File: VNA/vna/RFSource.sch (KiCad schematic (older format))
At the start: 15 parts, among them U4 AD9851, X1 30MHz

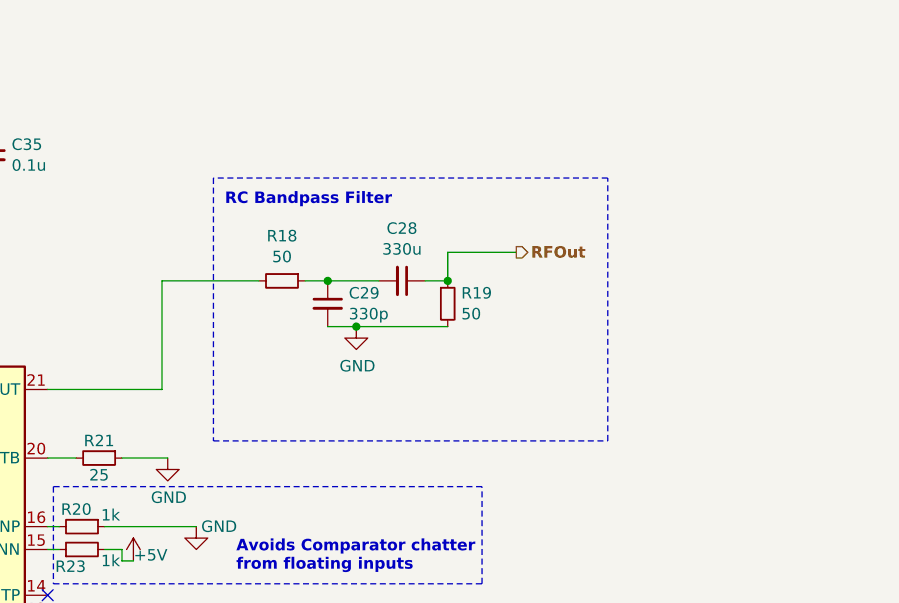
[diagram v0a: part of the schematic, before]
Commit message: v0.1 completed, producing gerbers
gerbers to be sent to jlc pcb pending their acceptance, they will be produced
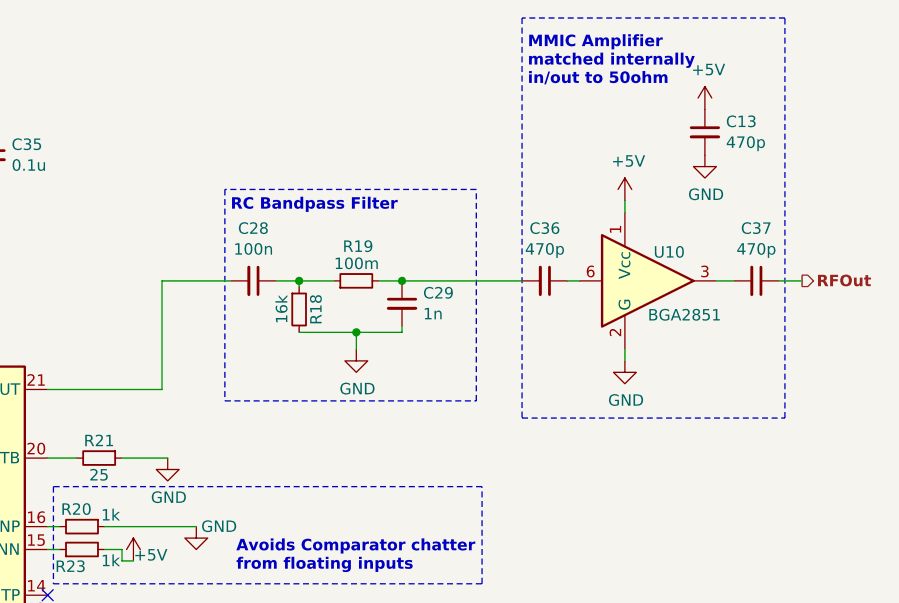
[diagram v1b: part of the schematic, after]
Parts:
- added C13, C36, C37: 470p, Capacitor_SMD:C_0805_2012Metric_Pad1.15x1.40mm_HandSolder, symbol Device:C_Small
- added U10: BGA2851, Package_TO_SOT_SMD:SOT-363_SC-70-6, symbol RF_Amplifier:BGA2851
- C28: value 330u -> 100n
- C29: value 330p -> 1n
- R18: value 50 -> 16k
- R19: value 50 -> 100m
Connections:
- net +5V: now also C13.1, U10.1 (Vcc)
- net GND: now also R18.2, C13.2, U10.2 (G), U10.4 (G), U10.5 (G); no longer R19.2
- net RFOut: now also C37.1; no longer C28.1, R19.1
- net at U4.21 (IOUT): now also C28.2; no longer R18.2
- new net: C28.1, R18.1, R19.1
- new net: C29.1, C36.2, R19.2
- new net: C37.2, U10.3
- new net: C36.1, U10.6
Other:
- note added: "MMIC Amplifier\nmatched internally\nin/out to 50ohm"
- moved on the sheet: C28, C29, R18, R19
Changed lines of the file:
@@
 Comment4 ""
 $EndDescr
-Text HLabel 6900 3400 2    50   Output ~ 10
+Text HLabel 8150 3525 2    50   Output ~ 10
 RFOut
 Text HLabel 3500 4900 0    50   Input ~ 10
@@
 Wire Wire Line
 	5350 4000 5350 3525
-Text Notes 5625 3200 0    50   ~ 10
+Text Notes 5650 3225 0    50   ~ 10
 RC Bandpass Filter
 $Comp
 L power:GND #PWR0102
 U 1 1 5D858459
-P 6200 3725
-F 0 "#PWR0102" H 6200 3475 50  0001 C CNN
-F 1 "GND" H 6205 3552 50  0000 C CNN
-F 2 "" H 6200 3725 50  0001 C CNN
-F 3 "" H 6200 3725 50  0001 C CNN
-	1    6200 3725
+P 6200 3825
+F 0 "#PWR0102" H 6200 3575 50  0001 C CNN
+F 1 "GND" H 6205 3652 50  0000 C CNN
+F 2 "" H 6200 3825 50  0001 C CNN
+F 3 "" H 6200 3825 50  0001 C CNN
+	1    6200 3825
 	1    0    0    -1
 $EndComp
@@
 L Device:R_Small R18
 U 1 1 5D90E295
-P 5875 3525
-F 0 "R18" V 5679 3525 50  0000 C CNN
-F 1 "50" V 5770 3525 50  0000 C CNN
-F 2 "Resistor_SMD:R_0805_2012Metric_Pad1.15x1.40mm_HandSolder" H 5875 3525 50  0001 C CNN
-F 3 "~" H 5875 3525 50  0001 C CNN
-	1    5875 3525
-	0    1    1    0
+P 5950 3650
+F 0 "R18" V 6025 3650 50  0000 C CNN
+F 1 "16k" V 5875 3650 50  0000 C CNN
+F 2 "Resistor_SMD:R_0805_2012Metric_Pad1.15x1.40mm_HandSolder" H 5950 3650 50  0001 C CNN
+F 3 "~" H 5950 3650 50  0001 C CNN
+	1    5950 3650
+	1    0    0    -1
 $EndComp
 $Comp
 L Device:R_Small R19
 U 1 1 5D90EC5A
-P 6600 3625
-F 0 "R19" H 6659 3671 50  0000 L CNN
-F 1 "50" H 6659 3580 50  0000 L CNN
-F 2 "Resistor_SMD:R_0805_2012Metric_Pad1.15x1.40mm_HandSolder" H 6600 3625 50  0001 C CNN
-F 3 "~" H 6600 3625 50  0001 C CNN
-	1    6600 3625
-	1    0    0    -1
+P 6200 3525
+F 0 "R19" V 6350 3450 50  0000 L CNN
+F 1 "100m" V 6275 3425 50  0000 L CNN
+F 2 "Resistor_SMD:R_0805_2012Metric_Pad1.15x1.40mm_HandSolder" H 6200 3525 50  0001 C CNN
+F 3 "~" H 6200 3525 50  0001 C CNN
+	1    6200 3525
+	0    -1   -1   0
 $EndComp
 $Comp
 L Device:C_Small C29
 U 1 1 5D90F928
-P 6075 3625
-F 0 "C29" H 6167 3671 50  0000 L CNN
-F 1 "330p" H 6167 3580 50  0000 L CNN
-F 2 "Capacitor_SMD:C_0805_2012Metric_Pad1.15x1.40mm_HandSolder" H 6075 3625 50  0001 C CNN
-F 3 "~" H 6075 3625 50  0001 C CNN
-	1    6075 3625
+P 6400 3625
+F 0 "C29" H 6492 3671 50  0000 L CNN
+F 1 "1n" H 6492 3580 50  0000 L CNN
+F 2 "Capacitor_SMD:C_0805_2012Metric_Pad1.15x1.40mm_HandSolder" H 6400 3625 50  0001 C CNN
+F 3 "~" H 6400 3625 50  0001 C CNN
+	1    6400 3625
 	1    0    0    -1
 $EndComp
@@
 L Device:C_Small C28
 U 1 1 5D9103E4
-P 6400 3525
-F 0 "C28" V 6171 3525 50  0000 C CNN
-F 1 "330u" V 6262 3525 50  0000 C CNN
-F 2 "Capacitor_SMD:C_0805_2012Metric_Pad1.15x1.40mm_HandSolder" H 6400 3525 50  0001 C CNN
-F 3 "~" H 6400 3525 50  0001 C CNN
-	1    6400 3525
+P 5750 3525
+F 0 "C28" V 5521 3525 50  0000 C CNN
+F 1 "100n" V 5612 3525 50  0000 C CNN
+F 2 "Capacitor_SMD:C_0805_2012Metric_Pad1.15x1.40mm_HandSolder" H 5750 3525 50  0001 C CNN
+F 3 "~" H 5750 3525 50  0001 C CNN
+	1    5750 3525
 	0    1    1    0
 $EndComp
-Wire Wire Line
-	5350 3525 5775 3525
-Wire Wire Line
-	5975 3525 6075 3525
-Wire Wire Line
-	6075 3525 6300 3525
-Connection ~ 6075 3525
-Wire Wire Line
-	6500 3525 6600 3525
-Wire Wire Line
-	6075 3725 6200 3725
-Connection ~ 6200 3725
-Wire Wire Line
-	6200 3725 6600 3725
-Wire Wire Line
-	6600 3525 6600 3400
-Wire Wire Line
-	6600 3400 6900 3400
-Connection ~ 6600 3525
-Wire Notes Line
-	5575 3075 5575 4225
-Wire Notes Line
-	5575 4225 7300 4225
-Wire Notes Line
-	7300 4225 7300 3075
-Wire Notes Line
-	7300 3075 5575 3075
 $Comp
 L Device:R_Small R20
@@
 Connection ~ 3550 2875
 Connection ~ 3550 3075
+$Comp
+L RF_Amplifier:BGA2851 U10
+U 1 1 5D98BDCA
+P 7475 3525
+F 0 "U10" H 7500 3650 50  0000 L CNN
+F 1 "BGA2851" H 7475 3375 50  0000 L CNN
+F 2 "Package_TO_SOT_SMD:SOT-363_SC-70-6" H 7425 2875 50  0001 C CNN
+F 3 "https://www.nxp.com/docs/en/data-sheet/BGA2851.pdf" H 7475 3525 50  0001 C CNN
+	1    7475 3525
+	1    0    0    -1
+$EndComp
+$Comp
+L power:+5V #PWR0120
+U 1 1 5D98ED21
+P 7375 3175
+F 0 "#PWR0120" H 7375 3025 50  0001 C CNN
+F 1 "+5V" H 7390 3348 50  0000 C CNN
+F 2 "" H 7375 3175 50  0001 C CNN
+F 3 "" H 7375 3175 50  0001 C CNN
+	1    7375 3175
+	1    0    0    -1
+$EndComp
+$Comp
+L power:GND #PWR0121
+U 1 1 5D98FE3B
+P 7375 3875
+F 0 "#PWR0121" H 7375 3625 50  0001 C CNN
+F 1 "GND" H 7380 3702 50  0000 C CNN
+F 2 "" H 7375 3875 50  0001 C CNN
+F 3 "" H 7375 3875 50  0001 C CNN
+	1    7375 3875
+	1    0    0    -1
+$EndComp
+Text Notes 6950 2675 0    50   ~ 10
+MMIC Amplifier\nmatched internally\nin/out to 50ohm
+Wire Wire Line
+	5350 3525 5650 3525
+Wire Wire Line
+	5850 3525 5950 3525
+Wire Wire Line
+	5950 3550 5950 3525
+Connection ~ 5950 3525
+Wire Wire Line
+	5950 3525 6100 3525
+Wire Wire Line
+	6300 3525 6400 3525
+Wire Wire Line
+	5950 3750 6200 3750
+Wire Wire Line
+	6400 3750 6400 3725
+Wire Wire Line
+	6200 3750 6200 3825
+Connection ~ 6200 3750
+Wire Wire Line
+	6200 3750 6400 3750
+Wire Notes Line
+	5625 3125 5625 4050
+Wire Notes Line
+	5625 4050 6725 4050
+Wire Notes Line
+	6725 4050 6725 3125
+Wire Notes Line
+	6725 3125 5625 3125
+Wire Wire Line
+	7375 3825 7375 3875
+Wire Wire Line
+	7375 3225 7375 3175
+$Comp
+L Device:C_Small C37
+U 1 1 5D9C2425
+P 7950 3525
+F 0 "C37" V 7721 3525 50  0000 C CNN
+F 1 "470p" V 7812 3525 50  0000 C CNN
+F 2 "Capacitor_SMD:C_0805_2012Metric_Pad1.15x1.40mm_HandSolder" H 7950 3525 50  0001 C CNN
+F 3 "~" H 7950 3525 50  0001 C CNN
+	1    7950 3525
+	0    1    1    0
+$EndComp
+$Comp
+L Device:C_Small C36
+U 1 1 5D9C3B15
+P 7025 3525
+F 0 "C36" V 6796 3525 50  0000 C CNN
+F 1 "470p" V 6887 3525 50  0000 C CNN
+F 2 "Capacitor_SMD:C_0805_2012Metric_Pad1.15x1.40mm_HandSolder" H 7025 3525 50  0001 C CNN
+F 3 "~" H 7025 3525 50  0001 C CNN
+	1    7025 3525
+	0    1    1    0
+$EndComp
+$Comp
+L Device:C_Small C13
+U 1 1 5D9C4738
+P 7725 2875
+F 0 "C13" H 7817 2921 50  0000 L CNN
+F 1 "470p" H 7817 2830 50  0000 L CNN
+F 2 "Capacitor_SMD:C_0805_2012Metric_Pad1.15x1.40mm_HandSolder" H 7725 2875 50  0001 C CNN
+F 3 "~" H 7725 2875 50  0001 C CNN
+	1    7725 2875
+	1    0    0    -1
+$EndComp
+Wire Wire Line
+	7125 3525 7175 3525
+Wire Wire Line
+	7775 3525 7850 3525
+Wire Wire Line
+	8050 3525 8150 3525
+Wire Notes Line
+	6925 4125 8075 4125
+Wire Notes Line
+	8075 4125 8075 2375
+Wire Notes Line
+	8075 2375 6925 2375
+Wire Notes Line
+	6925 2375 6925 4125
+Wire Wire Line
+	6400 3525 6925 3525
+Connection ~ 6400 3525
+$Comp
+L power:GND #PWR0122
+U 1 1 5D9DDA37
+P 7725 2975
+F 0 "#PWR0122" H 7725 2725 50  0001 C CNN
+F 1 "GND" H 7730 2802 50  0000 C CNN
+F 2 "" H 7725 2975 50  0001 C CNN
+F 3 "" H 7725 2975 50  0001 C CNN
+	1    7725 2975
+	1    0    0    -1
+$EndComp
+$Comp
+L power:+5V #PWR0123
+U 1 1 5D9DE892
+P 7725 2775
+F 0 "#PWR0123" H 7725 2625 50  0001 C CNN
+F 1 "+5V" H 7740 2948 50  0000 C CNN
+F 2 "" H 7725 2775 50  0001 C CNN
+F 3 "" H 7725 2775 50  0001 C CNN
+	1    7725 2775
+	1    0    0    -1
+$EndComp
 $EndSCHEMATC
